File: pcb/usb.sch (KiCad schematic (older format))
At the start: 9 parts, among them J600 USB_B_Micro, U100 LPC5500, U600 USBLC6-2SC6

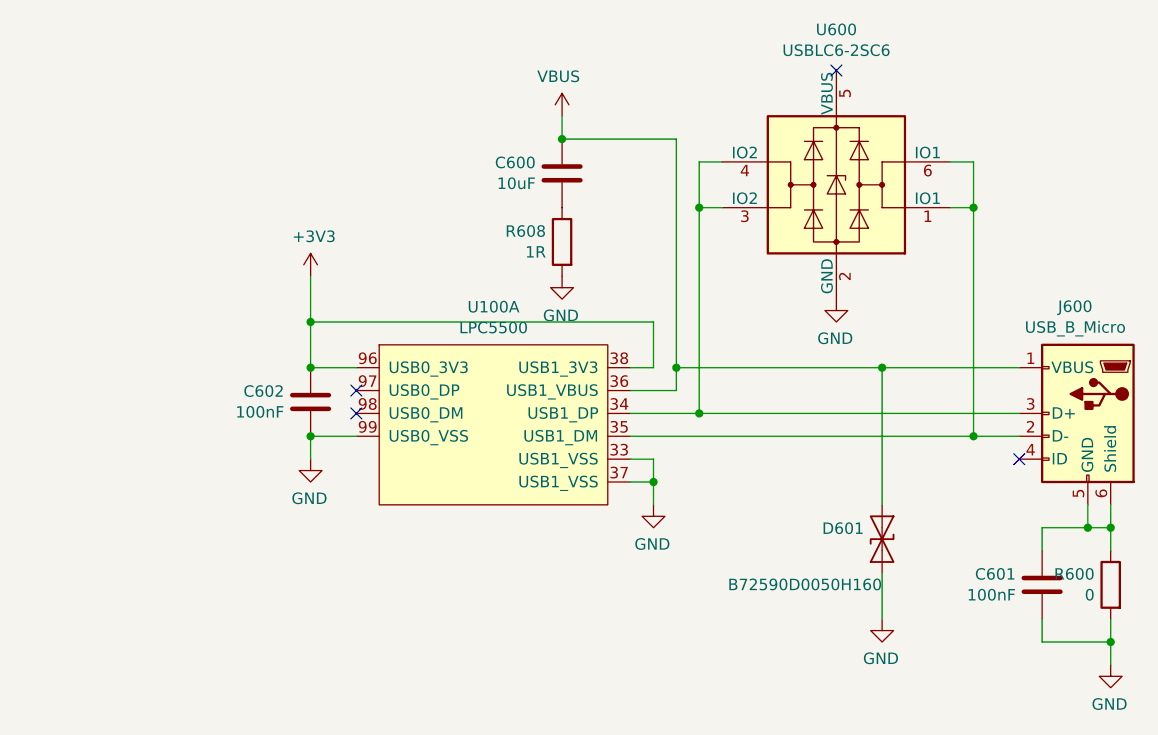
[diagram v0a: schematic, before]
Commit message: pcb: rev 0.1
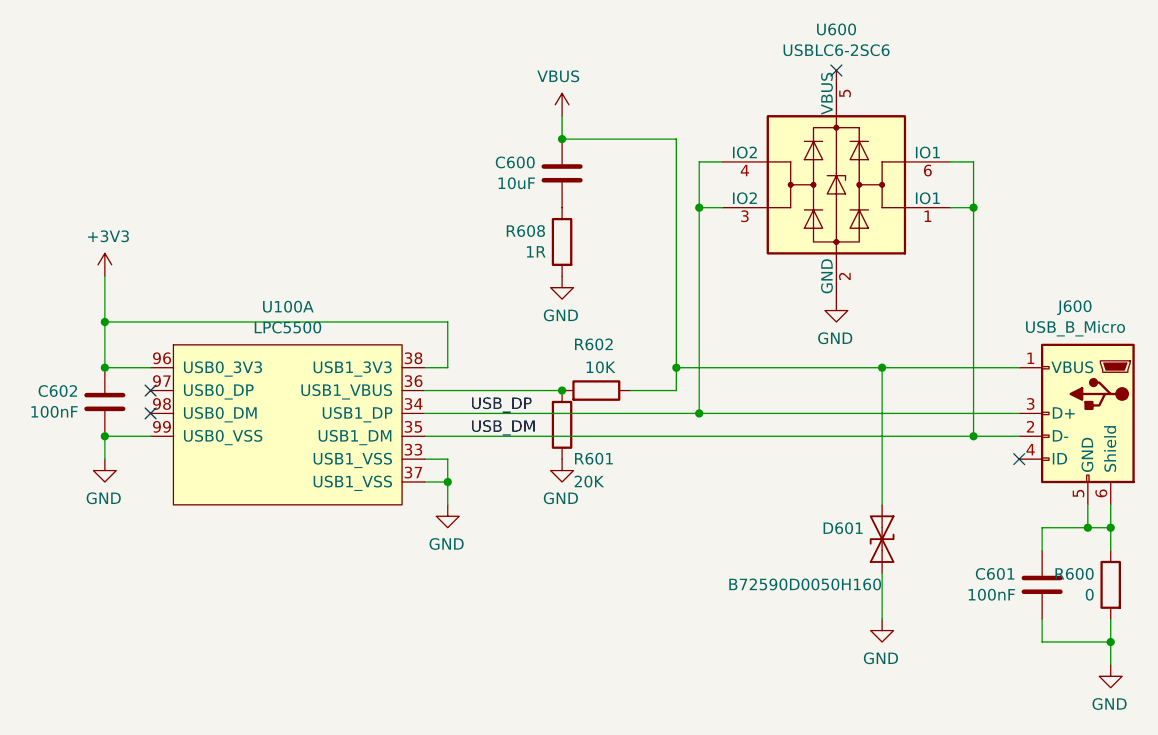
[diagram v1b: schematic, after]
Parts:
- added R601: 20K, Resistor_SMD:R_0603_1608Metric, symbol Device:R
- added R602: 10K, Resistor_SMD:R_0603_1608Metric, symbol Device:R
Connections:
- net GND: now also R601.1
- net VBUS: now also R602.1; no longer U100.36 (USB1_VBUS)
- net USB_DM: now reaches J600.2 (D-), U100.35 (USB1_DM), U600.1 (IO1), U600.6 (IO1)
- net USB_DP: now reaches J600.3 (D+), U100.34 (USB1_DP), U600.3 (IO2), U600.4 (IO2)
- new net: R601.2, R602.2, U100.36 (USB1_VBUS)
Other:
- moved on the sheet: C602, U100A
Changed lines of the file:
@@
 L power:GND #PWR0294
 U 1 1 5C99627A
-P 4200 4500
-F 0 "#PWR0294" H 4200 4250 50  0001 C CNN
-F 1 "GND" H 4205 4327 50  0000 C CNN
-F 2 "" H 4200 4500 50  0001 C CNN
-F 3 "" H 4200 4500 50  0001 C CNN
-	1    4200 4500
+P 3300 4500
+F 0 "#PWR0294" H 3300 4250 50  0001 C CNN
+F 1 "GND" H 3305 4327 50  0000 C CNN
+F 2 "" H 3300 4500 50  0001 C CNN
+F 3 "" H 3300 4500 50  0001 C CNN
+	1    3300 4500
 	-1   0    0    -1
 $EndComp
@@
 Connection ~ 7100 4400
 Wire Wire Line
-	7100 4400 5600 4400
-Wire Wire Line
 	7000 3400 7100 3400
 Connection ~ 7100 3400
@@
 	5900 3200 5900 3400
 Connection ~ 5900 4300
-Wire Wire Line
-	5900 4300 5600 4300
 Wire Wire Line
 	6000 3400 5900 3400
@@
 L symbols:LPC5500 U100
 U 1 1 5D749DD3
-P 5000 4300
-F 0 "U100" H 5000 4765 50  0000 C CNN
-F 1 "LPC5500" H 5000 4674 50  0000 C CNN
-F 2 "Package_QFP:TQFP-100-1EP_14x14mm_P0.5mm_EP5x5mm_ThermalVias" H 5000 4700 50  0001 C CNN
-F 3 "" H 4900 4350 50  0001 C CNN
-	1    5000 4300
+P 4100 4300
+F 0 "U100" H 4100 4765 50  0000 C CNN
+F 1 "LPC5500" H 4100 4674 50  0000 C CNN
+F 2 "Package_QFP:TQFP-100-1EP_14x14mm_P0.5mm_EP5x5mm_ThermalVias" H 4100 4700 50  0001 C CNN
+F 3 "" H 4000 4350 50  0001 C CNN
+	1    4100 4300
 	1    0    0    -1
 $EndComp
@@
 NoConn ~ 7300 4500
 $Comp
-L power:GND #PWR?
+L power:GND #PWR0153
 U 1 1 5D75956E
-P 5700 4700
-F 0 "#PWR?" H 5700 4450 50  0001 C CNN
-F 1 "GND" H 5705 4527 50  0000 C CNN
-F 2 "" H 5700 4700 50  0001 C CNN
-F 3 "" H 5700 4700 50  0001 C CNN
-	1    5700 4700
-	-1   0    0    -1
-$EndComp
-Wire Wire Line
-	5600 4500 5700 4500
-Wire Wire Line
-	5700 4500 5700 4600
-Wire Wire Line
-	5600 4600 5700 4600
-Connection ~ 5700 4600
-Wire Wire Line
-	5700 4600 5700 4700
+P 4800 4700
+F 0 "#PWR0153" H 4800 4450 50  0001 C CNN
+F 1 "GND" H 4805 4527 50  0000 C CNN
+F 2 "" H 4800 4700 50  0001 C CNN
+F 3 "" H 4800 4700 50  0001 C CNN
+	1    4800 4700
+	-1   0    0    -1
+$EndComp
+Wire Wire Line
+	4700 4500 4800 4500
+Wire Wire Line
+	4800 4500 4800 4600
+Wire Wire Line
+	4700 4600 4800 4600
+Connection ~ 4800 4600
+Wire Wire Line
+	4800 4600 4800 4700
 Wire Wire Line
 	5300 3100 5800 3100
@@
 Connection ~ 5300 3100
 Wire Wire Line
-	4200 4400 4200 4500
-NoConn ~ 4400 4200
-NoConn ~ 4400 4300
-$Comp
-L power:+3V3 #PWR?
+	3300 4400 3300 4500
+NoConn ~ 3500 4200
+NoConn ~ 3500 4300
+$Comp
+L power:+3V3 #PWR0154
 U 1 1 5D76C848
-P 4200 3700
-F 0 "#PWR?" H 4200 3550 50  0001 C CNN
-F 1 "+3V3" H 4215 3873 50  0000 C CNN
-F 2 "" H 4200 3700 50  0001 C CNN
-F 3 "" H 4200 3700 50  0001 C CNN
-	1    4200 3700
+P 3300 3700
+F 0 "#PWR0154" H 3300 3550 50  0001 C CNN
+F 1 "+3V3" H 3315 3873 50  0000 C CNN
+F 2 "" H 3300 3700 50  0001 C CNN
+F 3 "" H 3300 3700 50  0001 C CNN
+	1    3300 3700
 	1    0    0    -1
 $EndComp
 $Comp
-L power:GND #PWR?
+L power:GND #PWR0155
 U 1 1 5D76D29D
 P 5300 3700
-F 0 "#PWR?" H 5300 3450 50  0001 C CNN
+F 0 "#PWR0155" H 5300 3450 50  0001 C CNN
 F 1 "GND" H 5305 3527 50  0000 C CNN
 F 2 "" H 5300 3700 50  0001 C CNN
@@
 $EndComp
 Wire Wire Line
-	5600 4100 5700 4100
-Wire Wire Line
-	4200 3900 4200 4100
-Wire Wire Line
-	5700 3900 5700 4100
-Wire Wire Line
-	4200 3700 4200 3900
-Connection ~ 4200 3900
+	4700 4100 4800 4100
+Wire Wire Line
+	3300 3900 3300 4100
+Wire Wire Line
+	4800 3900 4800 4100
+Wire Wire Line
+	3300 3700 3300 3900
+Connection ~ 3300 3900
 $Comp
 L Device:C C602
 U 1 1 5D85A4D4
-P 4200 4250
-F 0 "C602" H 4315 4296 50  0000 L CNN
-F 1 "100nF" H 4315 4205 50  0000 L CNN
-F 2 "Capacitor_SMD:C_0402_1005Metric" H 4238 4100 50  0001 C CNN
-F 3 "~" H 4200 4250 50  0001 C CNN
-	1    4200 4250
-	-1   0    0    -1
-$EndComp
-Wire Wire Line
-	4200 4100 4400 4100
-Connection ~ 4200 4100
-Wire Wire Line
-	4200 4400 4400 4400
-Connection ~ 4200 4400
-Wire Wire Line
-	4200 3900 5700 3900
+P 3300 4250
+F 0 "C602" H 3415 4296 50  0000 L CNN
+F 1 "100nF" H 3415 4205 50  0000 L CNN
+F 2 "Capacitor_SMD:C_0402_1005Metric" H 3338 4100 50  0001 C CNN
+F 3 "~" H 3300 4250 50  0001 C CNN
+	1    3300 4250
+	-1   0    0    -1
+$EndComp
+Wire Wire Line
+	3300 4100 3500 4100
+Connection ~ 3300 4100
+Wire Wire Line
+	3300 4400 3500 4400
+Connection ~ 3300 4400
+Wire Wire Line
+	3300 3900 4800 3900
+Wire Wire Line
+	4700 4300 5900 4300
+Wire Wire Line
+	4700 4400 7100 4400
+Text Label 4900 4300 0    50   ~ 0
+USB_DP
+Text Label 4900 4400 0    50   ~ 0
+USB_DM
+$Comp
+L Device:R R602
+U 1 1 5D867F2F
+P 5450 4200
+F 0 "R602" V 5650 4100 50  0000 L CNN
+F 1 "10K" V 5550 4150 50  0000 L CNN
+F 2 "Resistor_SMD:R_0603_1608Metric" V 5380 4200 50  0001 C CNN
+F 3 "~" H 5450 4200 50  0001 C CNN
+	1    5450 4200
+	0    1    -1   0
+$EndComp
+$Comp
+L Device:R R601
+U 1 1 5D8690B6
+P 5300 4350
+F 0 "R601" H 5350 4500 50  0000 L CNN
+F 1 "20K" H 5350 4600 50  0000 L CNN
+F 2 "Resistor_SMD:R_0603_1608Metric" V 5230 4350 50  0001 C CNN
+F 3 "~" H 5300 4350 50  0001 C CNN
+	1    5300 4350
+	1    0    0    1
+$EndComp
+$Comp
+L power:GND #PWR0158
+U 1 1 5D869EE7
+P 5300 4500
+F 0 "#PWR0158" H 5300 4250 50  0001 C CNN
+F 1 "GND" H 5305 4327 50  0000 C CNN
+F 2 "" H 5300 4500 50  0001 C CNN
+F 3 "" H 5300 4500 50  0001 C CNN
+	1    5300 4500
+	-1   0    0    -1
+$EndComp
+Wire Wire Line
+	4700 4200 5300 4200
+Connection ~ 5300 4200
 $EndSCHEMATC
